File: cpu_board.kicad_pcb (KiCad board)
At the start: 4 copper layers, 73 x 58 mm, 63 parts, among them J1 Conn_01x13, J10 Conn_02x12_Odd_Even, J11 Conn_02x12_Odd_Even, J12 Conn_02x12_Odd_Even, J13 Conn_02x12_Odd_Even, J14 Conn_02x12_Odd_Even, J15 Conn_02x12_Odd_Even, J2 Conn_02x05_Odd_Even, J3 Conn_02x12_Odd_Even, J4 Conn_01x13, J5 Conn_02x12_Odd_Even, J6 Conn_02x12_Odd_Even, J7 Conn_02x12_Odd_Even, J8 Conn_02x12_Odd_Even, J9 Conn_02x12_Odd_Even, U1 74HC191, U2 74HC191, U3 74HC191, U4 74HC245, U5 74HC245, U6 74HC02, U7 74HC08

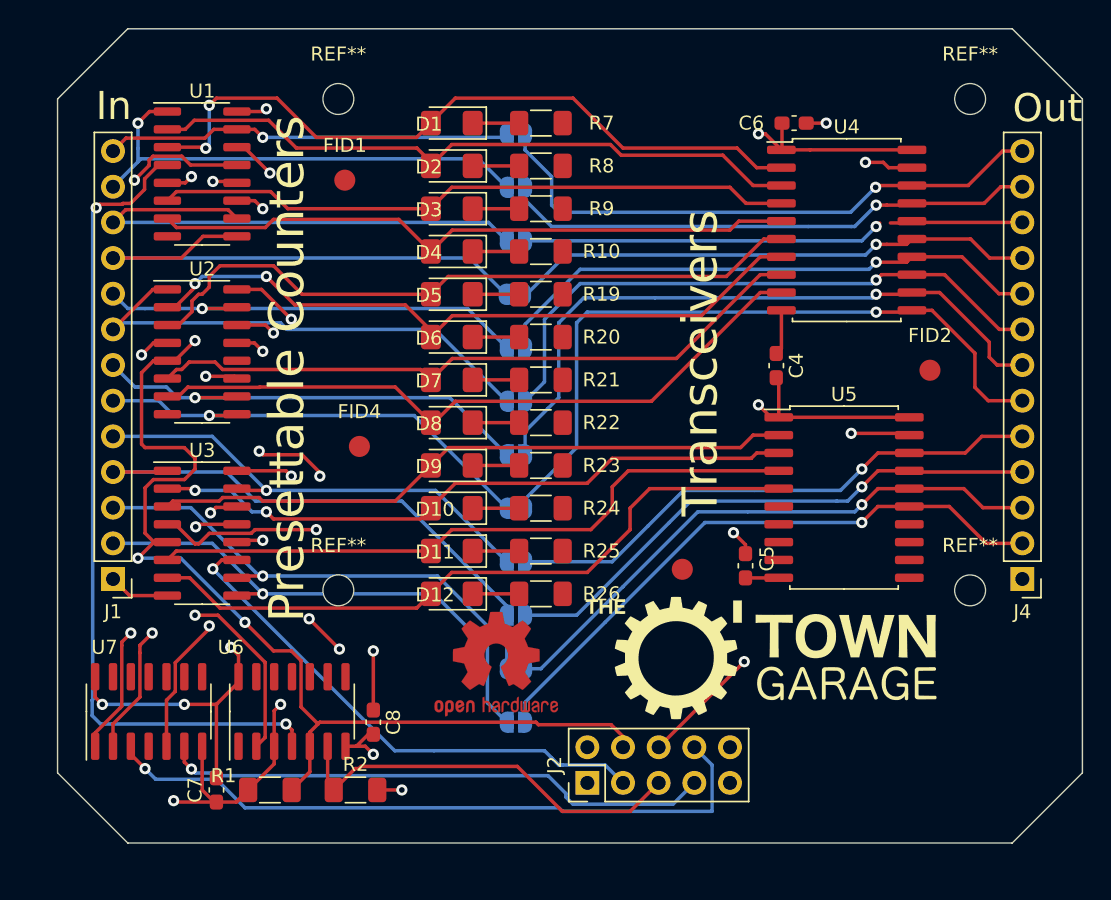
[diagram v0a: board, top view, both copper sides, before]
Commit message: routed and pretty
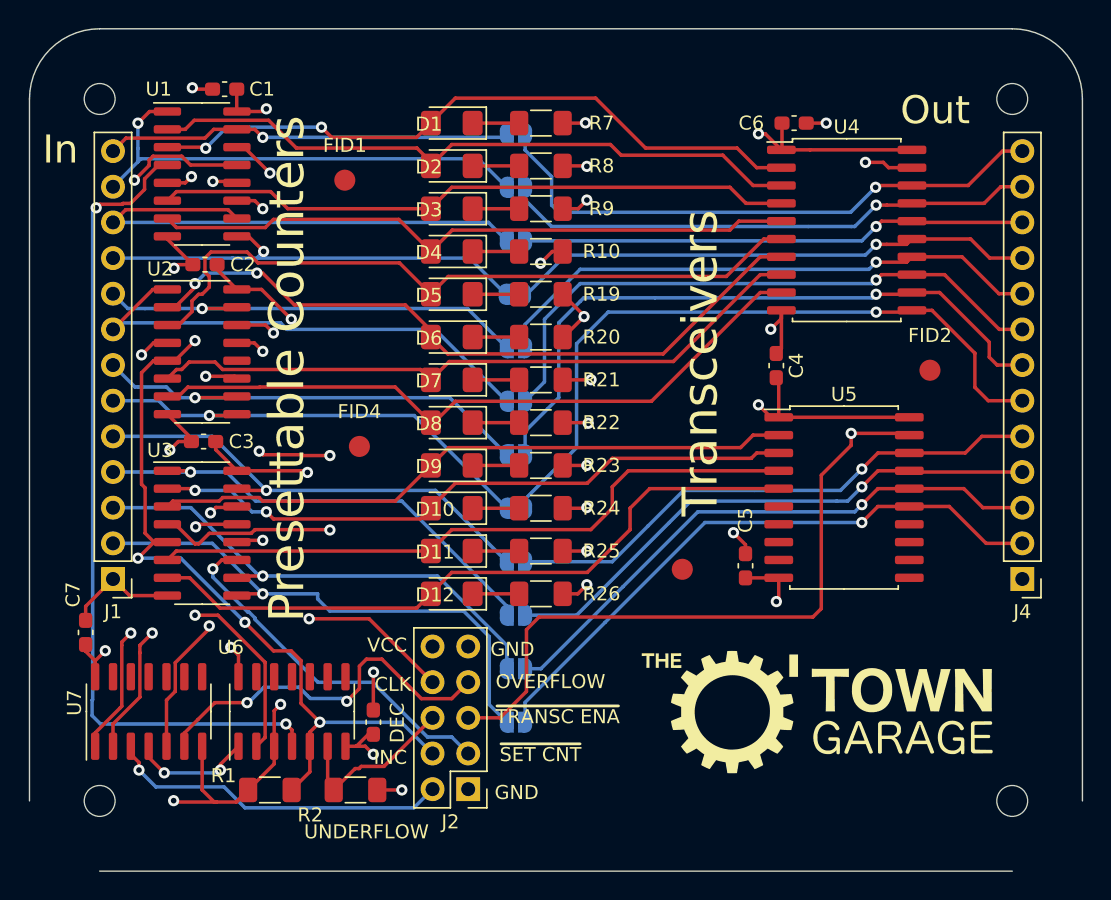
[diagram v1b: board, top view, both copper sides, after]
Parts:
- removed the REF** at (81.2, 95.2)
- added C1: 100nF, Capacitor_SMD:C_0603_1608Metric_Pad1.08x0.95mm_HandSolder, F.Cu at (61.9, 54.3)
- added C2: 100nF, Capacitor_SMD:C_0603_1608Metric_Pad1.08x0.95mm_HandSolder, F.Cu at (60.5, 66.8)
- added C3: 100nF, Capacitor_SMD:C_0603_1608Metric_Pad1.08x0.95mm_HandSolder, F.Cu at (60.4, 79.4)
- moved REF** 22.7 mm to (53.0, 105.0)
- moved REF** 17.0 mm to (53.0, 55.0)
- moved REF** 15.3 mm to (118.0, 105.0)
- moved C7 14.6 mm to (52.0, 93.0)
- moved J2 8.50 mm to (79.2, 104.2), turned to 180 degrees
- moved ? 5.55 mm to (104.0, 98.6)
- moved REF** 3.00 mm to (118.0, 55.0)
- turned C8 to 90 degrees
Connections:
- J2 pad 2: CLK -> /Presettable counters/UNDERFLOW
- J2 pad 5: /Presettable counters/~{INC}/DEC -> /Presettable counters/~{TRANSC_ENA}
- J2 pad 6: /Presettable counters/~{TRANSC_ENA} -> /Presettable counters/~{INC}/DEC
- J2 pad 8: /Presettable counters/UNDERFLOW -> CLK
- U2 pad 15: unconnected-(U2-Pad15) -> /Presettable counters/IN_4
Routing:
- net GND: track 30.4 -> 74.1 mm, vias 4 -> 21
- net /Presettable counters/UNDERFLOW: track 48.8 -> 24.5 mm
- net /Presettable counters/INC/~{DEC}: track 88.3 -> 68.0 mm, vias 4 -> 5
- net /Presettable counters/~{INC}/DEC: track 29.3 -> 12.5 mm
- net /Presettable counters/~{TRANSC_ENA}: track 55.4 -> 71.7 mm, vias 3 -> 2
- net CLK: track 70.0 -> 56.8 mm, vias 5 -> 4
- net /Presettable counters/OVERFLOW: track 39.5 -> 26.8 mm, vias 1 -> 2
- net /Presettable counters/~{SET_CNT}: track 70.7 -> 59.2 mm
- net VCC: track 202.4 -> 193.3 mm, vias 11 -> 9
- net Net-(U6-Pad1): track 0.83 -> 8.67 mm, vias 0 -> 2
- net /Presettable counters/IN_3: track 38.5 -> 32.0 mm, vias 0 -> 1
- net /Presettable counters/CNT_0: track 51.3 -> 47.9 mm
- net /Presettable counters/~{RCO_2}: track 30.0 -> 32.4 mm
- net /Presettable counters/IN_9: track 36.6 -> 34.3 mm, vias 0 -> 1
- net /Presettable counters/CNT_4: track 48.9 -> 50.9 mm
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- added copper zone on In2.Cu, net GND
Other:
- board size 73 x 58 mm -> 75 x 60 mm
- board text added: "CLK"
- board text added: "DEC"
- board text added: "GND"
- board text added: "INC"
- board text added: "OVERFLOW"
- board text added: "UNDERFLOW"
- board text added: "VCC"
- board text added: "~{SET CNT}"
- board text added: "~{TRANSC ENA}"
